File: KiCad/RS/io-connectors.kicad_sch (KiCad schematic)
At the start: 50 parts, among them J3 ST-LINK, J4 SPI, J5 MODEM, J6 I2C, Q3 BC817, Q4 BC817, Q5 P60V/2A, Q6 P60V/2A, Q7 BC817, Q8 BC817, U6 TLP185, U7 TLP185

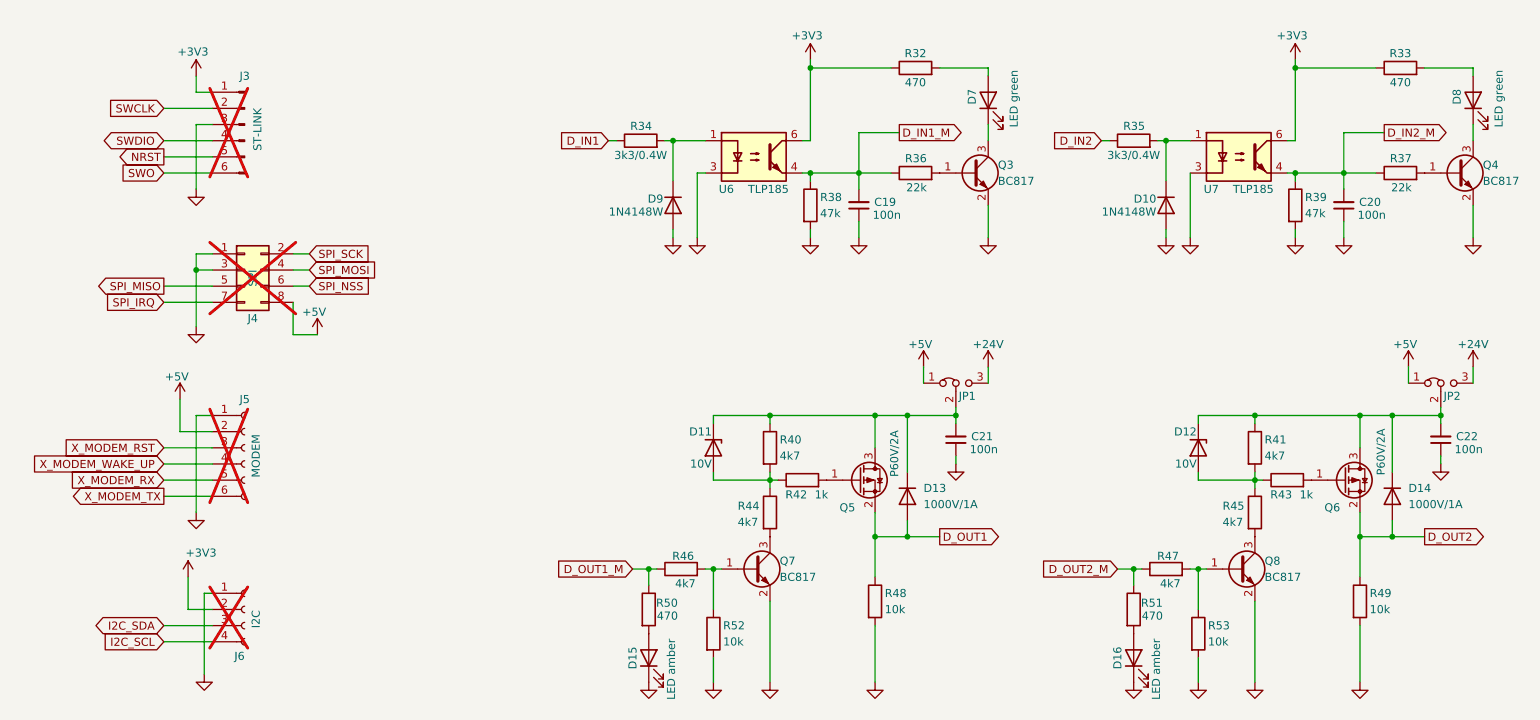
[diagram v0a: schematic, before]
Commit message: FIX: Schematics + BOM.
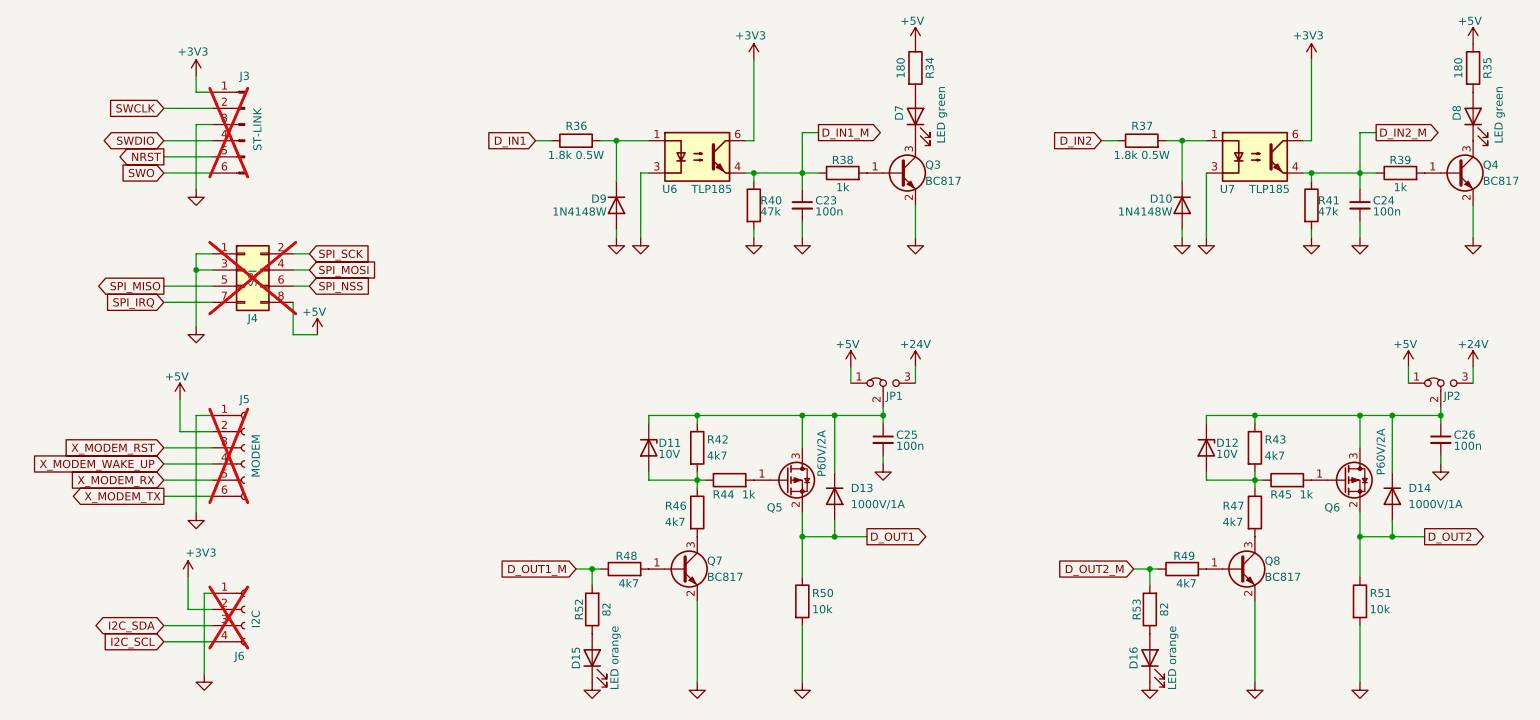
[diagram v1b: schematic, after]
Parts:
- removed C19, C20, C21, C22: 100n, Capacitor_SMD:C_0805_2012Metric_Pad1.18x1.45mm_HandSolder, symbol Device:C_Small
- removed R33, R50, R51: 470, Resistor_SMD:R_0805_2012Metric_Pad1.20x1.40mm_HandSolder, symbol Device:R
- added C23, C24, C25, C26: 100n, Capacitor_SMD:C_0402_1005Metric_Pad0.74x0.62mm_HandSolder, symbol Device:C_Small
- added R41: 47k, Resistor_SMD:R_0402_1005Metric_Pad0.72x0.64mm_HandSolder, symbol Device:R
- D11, D12: footprint Diode_SMD:D_MiniMELF -> Diode_SMD:D_SOD-323
- D15, D16: value LED amber -> LED orange; Mfg Part # B1701UY--20D000214U1930 -> LO R976-PS-1-0-20-R18; URL https://www.digikey.pl/en/products/detail/harvatek-corporat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 -> https://www.digikey.pl/en/products/detail/ams-osram-ag/LO-R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; URL2 CL-270HR-C -> (none)
- D7, D8: Mfg Part # B1701NG--20D000314U1930 -> LG R971-KN-1-0-20-R18; URL https://www.digikey.pl/en/products/detail/harvatek-corporat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 -> https://www.digikey.pl/en/products/detail/ams-osram-ag/LG-R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; URL2 CL-270HR-C -> (none)
- R34: renamed from R32; value 470 -> 180; footprint Resistor_SMD:R_0805_2012Metric_Pad1.20x1.40mm_HandSolder -> Resistor_SMD:R_0402_1005Metric_Pad0.72x0.64mm_HandSolder; Mfg Part # CR0805JB470RS1 -> CR0402-FX-1800GLF; URL https://www.digikey.pl/en/products/detail/nextgen-component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 -> https://www.digikey.pl/en/products/detail/bourns-inc/CR0402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
- R35: value 3k3/0.4W -> 180; footprint Resistor_SMD:R_0805_2012Metric_Pad1.20x1.40mm_HandSolder -> Resistor_SMD:R_0402_1005Metric_Pad0.72x0.64mm_HandSolder; Mfg Part # ESR10EZPJ332 -> CR0402-FX-1800GLF; URL https://www.digikey.pl/en/products/detail/rohm-semiconducto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 -> https://www.digikey.pl/en/products/detail/bourns-inc/CR0402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
- R36: renamed from R34; value 3k3/0.4W -> 1.8k 0.5W; footprint Resistor_SMD:R_0805_2012Metric_Pad1.20x1.40mm_HandSolder -> Resistor_SMD:R_0603_1608Metric_Pad0.98x0.95mm_HandSolder; Mfg Part # ESR10EZPJ332 -> SG73P1JTTD182J; URL https://www.digikey.pl/en/products/detail/rohm-semiconducto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 -> https://www.digikey.pl/en/products/detail/koa-speer-electro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
- R37: value 22k -> 1.8k 0.5W; footprint Resistor_SMD:R_0805_2012Metric_Pad1.20x1.40mm_HandSolder -> Resistor_SMD:R_0603_1608Metric_Pad0.98x0.95mm_HandSolder; Mfg Part # SG73G2ATTD2202D -> SG73P1JTTD182J; URL https://www.digikey.pl/en/products/detail/koa-speer-electronics-inc/SG73G2ATTD2202D/16823265 -> https://www.digikey.pl/en/products/detail/koa-speer-electronics-inc/SG73P1JTTD182J/10189924
- R38: renamed from R36; value 22k -> 1k; footprint Resistor_SMD:R_0805_2012Metric_Pad1.20x1.40mm_HandSolder -> Resistor_SMD:R_0402_1005Metric_Pad0.72x0.64mm_HandSolder; Mfg Part # SG73G2ATTD2202D -> RNCP0402FTD1K00; URL https://www.digikey.pl/en/products/detail/koa-speer-electro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 -> https://www.digikey.pl/en/products/detail/stackpole-electro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
- R39: value 47k -> 1k; footprint Resistor_SMD:R_0805_2012Metric_Pad1.20x1.40mm_HandSolder -> Resistor_SMD:R_0402_1005Metric_Pad0.72x0.64mm_HandSolder; Mfg Part # SFR10EZPJ473 -> RNCP0402FTD1K00; URL https://www.digikey.pl/en/products/detail/rohm-semiconducto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 -> https://www.digikey.pl/en/products/detail/stackpole-electro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
- R40: renamed from R38; footprint Resistor_SMD:R_0805_2012Metric_Pad1.20x1.40mm_HandSolder -> Resistor_SMD:R_0402_1005Metric_Pad0.72x0.64mm_HandSolder; Mfg Part # SFR10EZPJ473 -> RT0402FRE1347KL; URL https://www.digikey.pl/en/products/detail/rohm-semiconducto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 -> https://www.digikey.pl/en/products/detail/yageo/RT0402FRE13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
- R44: renamed from R42; footprint Resistor_SMD:R_0805_2012Metric_Pad1.20x1.40mm_HandSolder -> Resistor_SMD:R_0402_1005Metric_Pad0.72x0.64mm_HandSolder; Mfg Part # CR0805JB1KS001 -> RNCP0402FTD1K00; URL https://www.digikey.pl/en/products/detail/vishay-dale/CRCW0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 -> https://www.digikey.pl/en/products/detail/stackpole-electro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
- R45: renamed from R43; footprint Resistor_SMD:R_0805_2012Metric_Pad1.20x1.40mm_HandSolder -> Resistor_SMD:R_0402_1005Metric_Pad0.72x0.64mm_HandSolder; Mfg Part # CR0805JB1KS001 -> RNCP0402FTD1K00; URL https://www.digikey.pl/en/products/detail/vishay-dale/CRCW0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 -> https://www.digikey.pl/en/products/detail/stackpole-electro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
- R52, R53: value 10k -> 82; Mfg Part # RMCF0402FT10K0 -> RT0402FRE0782RL; URL https://www.digikey.pl/en/products/detail/stackpole-electro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 -> https://www.digikey.pl/en/products/detail/yageo/RT0402FRE07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
- U6, U7: Mfg Part # (none) -> TLP185(GB-TPL,SE; URL (none) -> https://www.digikey.pl/en/products/detail/toshiba-semicondu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
- renumbered R40 to R42, R41 to R43, R44 to R46, R45 to R47, R46 to R48, R47 to R49, R48 to R50, R49 to R51
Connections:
- net +3V3: no longer R34.1
- net +5V: now also R34.1, R35.1
- net D_IN1_M: now also C23.1
- net D_IN2: now also R37.1; no longer R35.1
- net D_IN2_M: now also C24.1, R41.1; no longer R37.1
- net D_OUT1_M: now also R52.2
- net D_OUT2_M: now also R53.2
- net GND: now also C23.2, C24.2, C25.2, C26.2, R41.2; no longer R39.2, R52.2, R53.2
- net at D10.1 (K), U7.1: now also R37.2; no longer R35.2
- net at D16.2 (A): now also R53.1
- net at Q4.1 (B): now also R39.2; no longer R37.2
- net at D12.1 (K), D14.1 (K), JP2.2 (C)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: now also C26.1
- net at D11.1 (K), D13.1 (K), JP1.2 (C)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: now also C25.1
- net at Q7.1 (B), R48.2: no longer R52.1
- net at D15.2 (A): now also R52.1
- net at Q8.1 (B), R49.2: no longer R53.1
- net at D8.2 (A): now also R35.2
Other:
- moved on the sheet: D10, D11, D13, D9, JP1, Q3, Q5, Q7, R34, R36, R38, R40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

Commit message: FIX: Everything. 1.0.
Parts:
- D13, D14: footprint Diode_SMD:D_SMA_Handsoldering -> CodeDog:D_SMA
- D15: Label (none) -> OUT1
- D16: Label (none) -> OUT2
- D7: Label (none) -> IN1
- D8: Label (none) -> IN2
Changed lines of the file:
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@@
 	(title_block
 		(title "Remote Sensor Module: Digital I/O Sheet")
-		(date "2026-07-25")
+		(date "2026-08-15")
 		(rev "0.1")
 		(company "CodeDog")
+		(comment 1 "(c)2026")
+		(comment 2 "All rights reserved")
 	)
 	(junction
@@
 			)
 		)
+		(property "Label" "OUT2"
+			(at 215.9 132.08 0)
+			(hide yes)
+			(show_name no)
+			(do_not_autoplace no)
+			(effects
+				(font
+					(size 1.27 1.27)
+				)
+			)
+		)
 		(pin "1"
 		)
@@
 			)
 		)
+		(property "Label" "IN2"
+			(at 266.7 46.99 0)
+			(hide yes)
+			(show_name no)
+			(do_not_autoplace no)
+			(effects
+				(font
+					(size 1.27 1.27)
+				)
+			)
+		)
 		(pin "1"
 		)
@@
 			)
 		)
+		(property "Label" "OUT1"
+			(at 128.27 132.08 0)
+			(hide yes)
+			(show_name no)
+			(do_not_autoplace no)
+			(effects
+				(font
+					(size 1.27 1.27)
+				)
+			)
+		)
 		(pin "1"
 		)
@@
 			)
 		)
+		(property "Label" "IN1"
+			(at 179.07 46.99 0)
+			(hide yes)
+			(show_name no)
+			(do_not_autoplace no)
+			(effects
+				(font
+					(size 1.27 1.27)
+				)
+			)
+		)
 		(pin "1"
 		)
@@
 			)
 		)
-		(property "Footprint" "Diode_SMD:D_SMA_Handsoldering"
+		(property "Footprint" "CodeDog:D_SMA"
 			(at 161.925 106.68 0)
 			(hide yes)
@@
 			)
 		)
-		(property "Footprint" "Diode_SMD:D_SMA_Handsoldering"
+		(property "Footprint" "CodeDog:D_SMA"
 			(at 249.555 106.68 0)
 			(hide yes)
